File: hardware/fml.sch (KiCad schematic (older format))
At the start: 11 parts, among them J1 midi_in, J2 midi_out, U1 Teensy3.6, U2 6N138

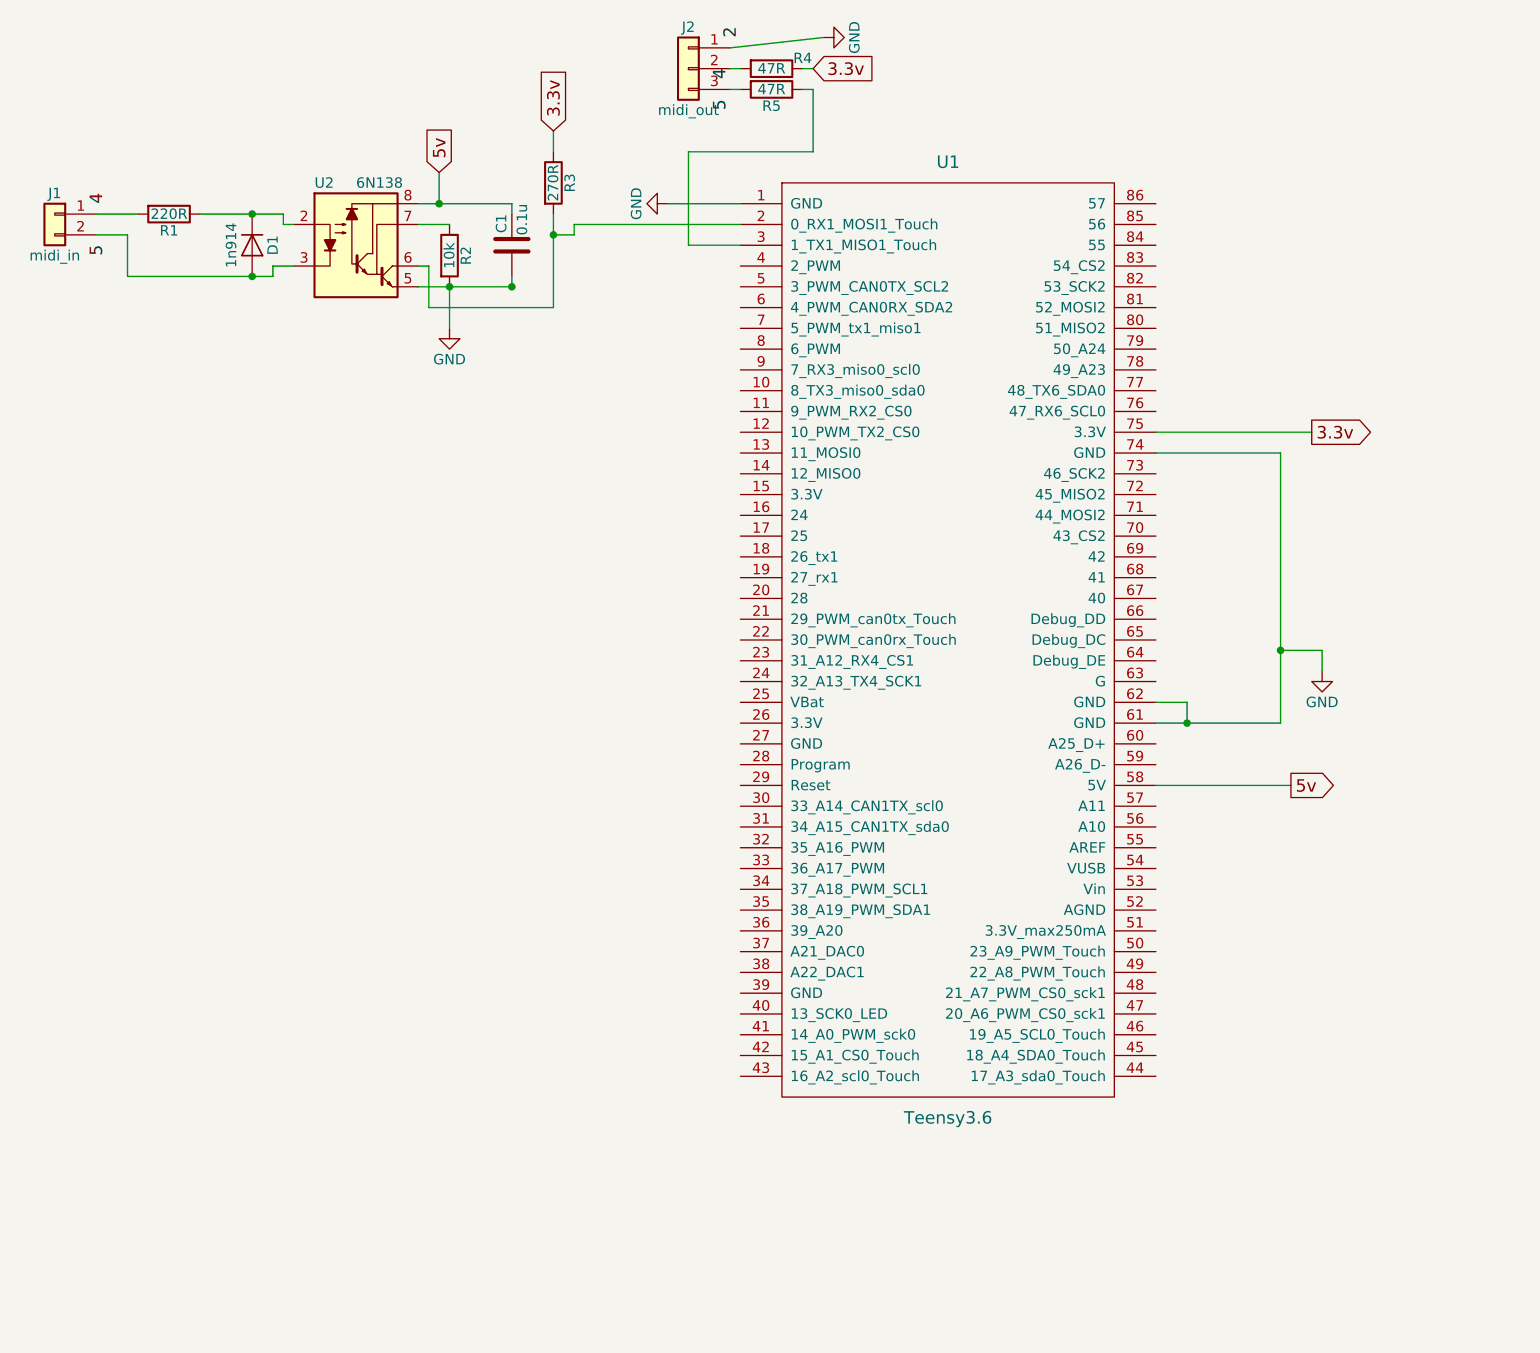
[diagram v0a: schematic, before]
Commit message: pcb updates
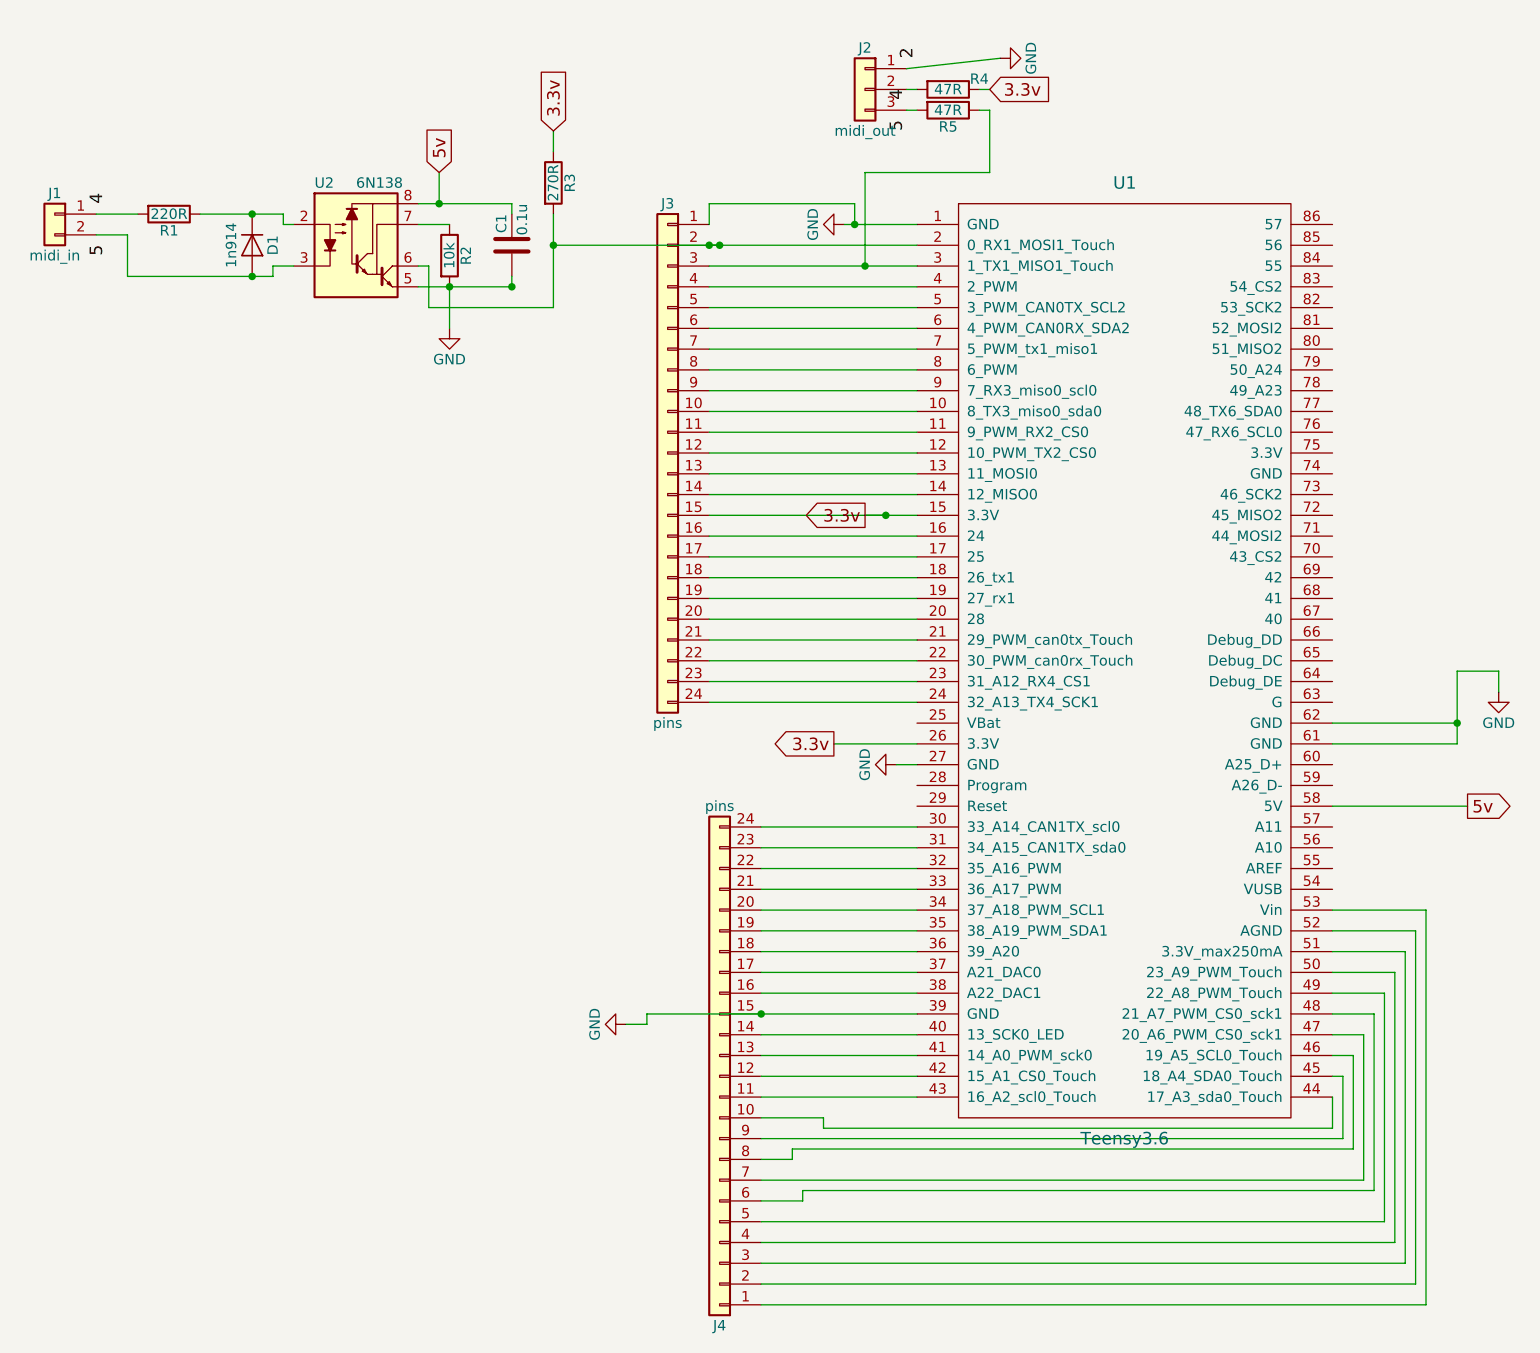
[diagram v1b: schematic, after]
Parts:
- added J3, J4: pins, Pin_Headers:Pin_Header_Straight_1x24_Pitch2.54mm, symbol Conn_01x24
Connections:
- net 3.3v: now also U1.15 (3.3V), U1.26 (3.3V), J3.15 (Pin_15); no longer U1.75 (3.3V)
- net GND: now also U1.27 (GND), U1.39 (GND), J3.1 (Pin_1), J4.15 (Pin_15); no longer U1.74 (GND)
- net at U1.10 (8_TX3_miso0_sda0): now also J3.10 (Pin_10)
- net at U1.11 (9_PWM_RX2_CS0): now also J3.11 (Pin_11)
- net at U1.12 (10_PWM_TX2_CS0): now also J3.12 (Pin_12)
- net at U1.13 (11_MOSI0): now also J3.13 (Pin_13)
- net at U1.14 (12_MISO0): now also J3.14 (Pin_14)
- net at U1.16 (24): now also J3.16 (Pin_16)
- net at U1.17 (25): now also J3.17 (Pin_17)
- net at U1.18 (26_tx1): now also J3.18 (Pin_18)
- net at U1.19 (27_rx1): now also J3.19 (Pin_19)
- net at R3.2, U1.2 (0_RX1_MOSI1_Touch), U2.6: now also J3.2 (Pin_2)
- net at U1.20 (28): now also J3.20 (Pin_20)
- net at U1.21 (29_PWM_can0tx_Touch): now also J3.21 (Pin_21)
- net at U1.22 (30_PWM_can0rx_Touch): now also J3.22 (Pin_22)
- net at U1.23 (31_A12_RX4_CS1): now also J3.23 (Pin_23)
- net at U1.24 (32_A13_TX4_SCK1): now also J3.24 (Pin_24)
- net at R5.1, U1.3 (1_TX1_MISO1_Touch): now also J3.3 (Pin_3)
- net at U1.30 (33_A14_CAN1TX_scl0): now also J4.24 (Pin_24)
- net at U1.31 (34_A15_CAN1TX_sda0): now also J4.23 (Pin_23)
- net at U1.32 (35_A16_PWM): now also J4.22 (Pin_22)
- net at U1.33 (36_A17_PWM): now also J4.21 (Pin_21)
- net at U1.34 (37_A18_PWM_SCL1): now also J4.20 (Pin_20)
- net at U1.35 (38_A19_PWM_SDA1): now also J4.19 (Pin_19)
- net at U1.36 (39_A20): now also J4.18 (Pin_18)
- net at U1.37 (A21_DAC0): now also J4.17 (Pin_17)
- net at U1.38 (A22_DAC1): now also J4.16 (Pin_16)
- net at U1.4 (2_PWM): now also J3.4 (Pin_4)
- net at U1.40 (13_SCK0_LED): now also J4.14 (Pin_14)
- net at U1.41 (14_A0_PWM_sck0): now also J4.13 (Pin_13)
- net at U1.42 (15_A1_CS0_Touch): now also J4.12 (Pin_12)
- net at U1.43 (16_A2_scl0_Touch): now also J4.11 (Pin_11)
- net at U1.44 (17_A3_sda0_Touch): now also J4.10 (Pin_10)
- net at U1.45 (18_A4_SDA0_Touch): now also J4.9 (Pin_9)
- net at U1.46 (19_A5_SCL0_Touch): now also J4.8 (Pin_8)
- net at U1.47 (20_A6_PWM_CS0_sck1): now also J4.7 (Pin_7)
- net at U1.48 (21_A7_PWM_CS0_sck1): now also J4.6 (Pin_6)
- net at U1.49 (22_A8_PWM_Touch): now also J4.5 (Pin_5)
- net at U1.5 (3_PWM_CAN0TX_SCL2): now also J3.5 (Pin_5)
- net at U1.50 (23_A9_PWM_Touch): now also J4.4 (Pin_4)
- net at U1.51 (3.3V_max250mA): now also J4.3 (Pin_3)
- net at U1.52 (AGND): now also J4.2 (Pin_2)
- net at U1.53 (Vin): now also J4.1 (Pin_1)
- net at U1.6 (4_PWM_CAN0RX_SDA2): now also J3.6 (Pin_6)
- net at U1.7 (5_PWM_tx1_miso1): now also J3.7 (Pin_7)
- net at U1.8 (6_PWM): now also J3.8 (Pin_8)
- net at U1.9 (7_RX3_miso0_scl0): now also J3.9 (Pin_9)
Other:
- moved on the sheet: J2, R4, R5, U1
